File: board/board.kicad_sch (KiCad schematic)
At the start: 23 parts, among them J1 port attiny, J10 BMS Bat +, J11 BMS Bat gnd, J12 BMS out -, J13 BMS in +5v, J14 BMS in gnd, J15 alim mp3 -, J17 next, J18 vol -, J2 Conn_01x02_Pin, J24 port 3-C265421, J3 alim mp3 +, J4 hp mp3, J5 step out - gnd, J6 step up out+, J7 step up in +, J8 step up in -, J9 BMS out +

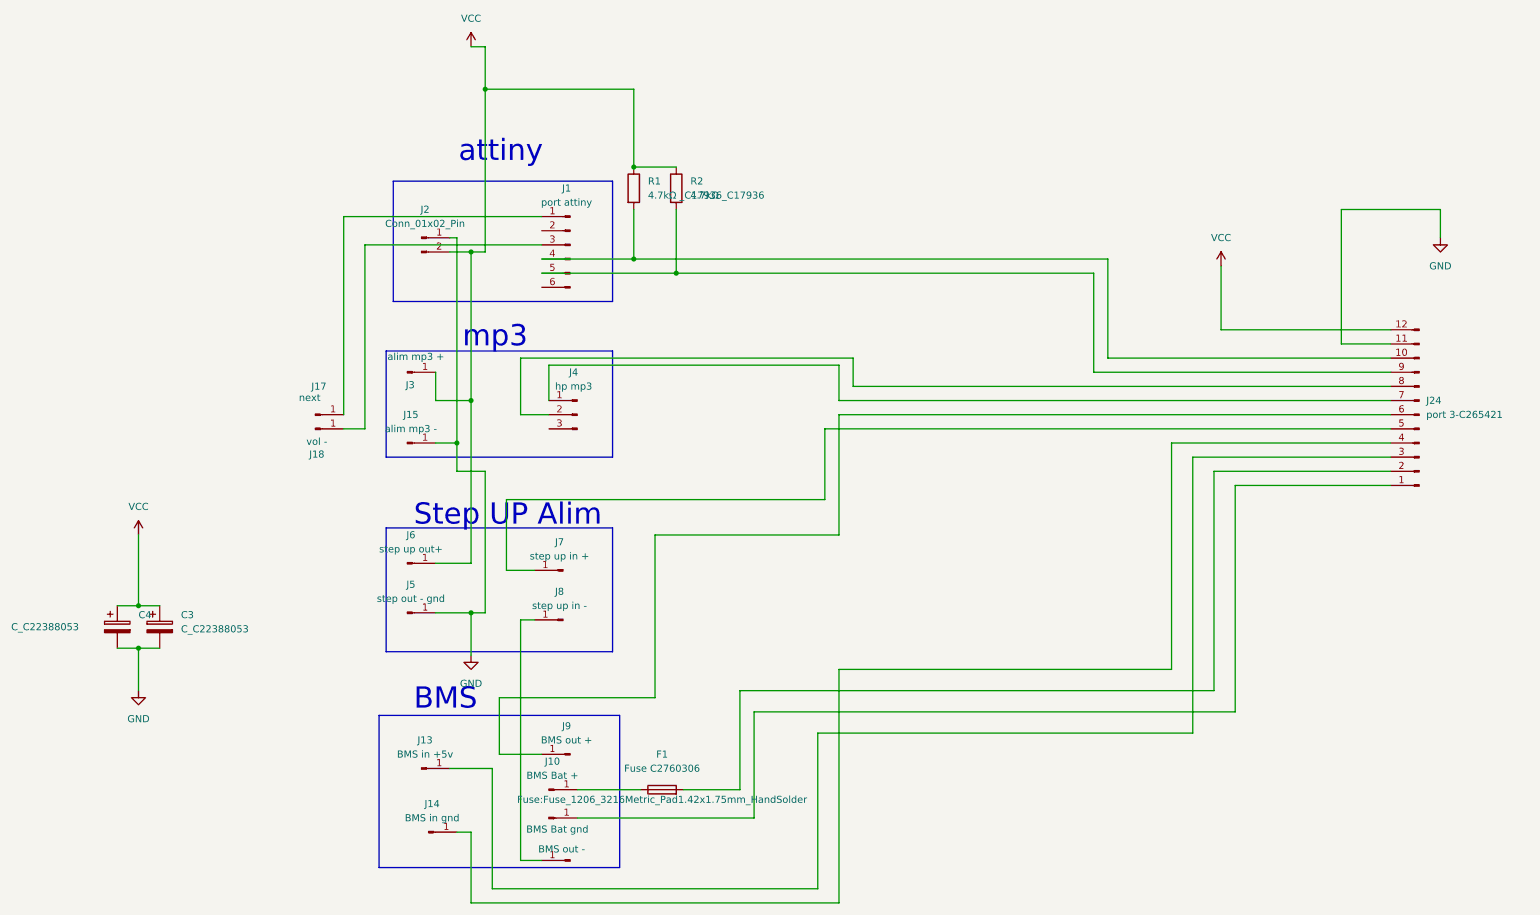
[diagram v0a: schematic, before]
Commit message: ajout etiquette global + plan de masse
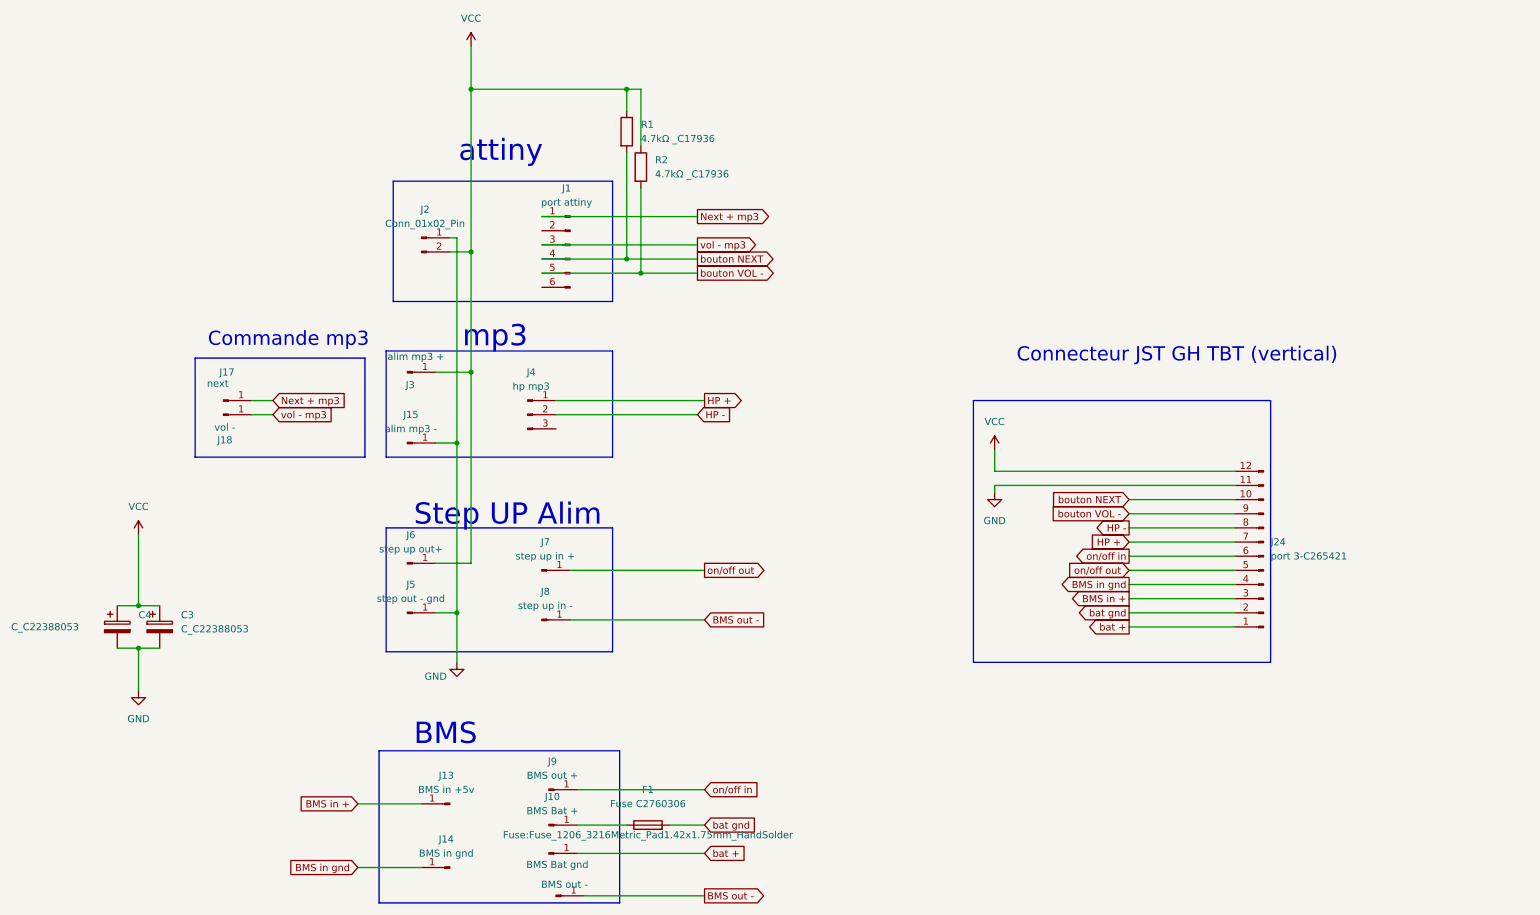
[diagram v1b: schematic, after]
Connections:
- net Next + mp3: now reaches J1.1 (Pin_1), J17.1 (Pin_1)
- net vol - mp3: now reaches J1.3 (Pin_3), J18.1 (Pin_1)
- net bouton NEXT: now reaches J1.4 (Pin_4), J24.10 (Pin_10), R1.2
- net bouton VOL -: now reaches J1.5 (Pin_5), J24.9 (Pin_9), R2.2
- net bat gnd: now reaches F1.2, J24.2 (Pin_2)
- net bat +: now reaches J11.1 (Pin_1), J24.1 (Pin_1)
- net BMS out -: now reaches J12.1 (Pin_1), J8.1 (Pin_1)
- net BMS in +: now reaches J13.1 (Pin_1), J24.3 (Pin_3)
- net BMS in gnd: now reaches J14.1 (Pin_1), J24.4 (Pin_4)
- net on/off out: now reaches J24.5 (Pin_5), J7.1 (Pin_1)
- net on/off in: now reaches J24.6 (Pin_6), J9.1 (Pin_1)
- net HP +: now reaches J24.7 (Pin_7), J4.1 (Pin_1)
- net HP -: now reaches J24.8 (Pin_8), J4.2 (Pin_2)
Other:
- note added: "Commande mp3"
- note added: "Connecteur JST GH TBT (vertical)"
- moved on the sheet: F1, J10, J13, J14, J17, J18, J24, J4, J7, J8, J9, R1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
